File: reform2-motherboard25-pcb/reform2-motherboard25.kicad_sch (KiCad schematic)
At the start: 44 parts, among them J15 Conn_01x33, J18 Conn_01x03_Male, J19 JTAG, J20 Conn_01x03_Male, SW3 SW_DIP_x01, SW5 SW_DIP_x04, SW6 SW_Push, U1 Nitrogen8M_SOM

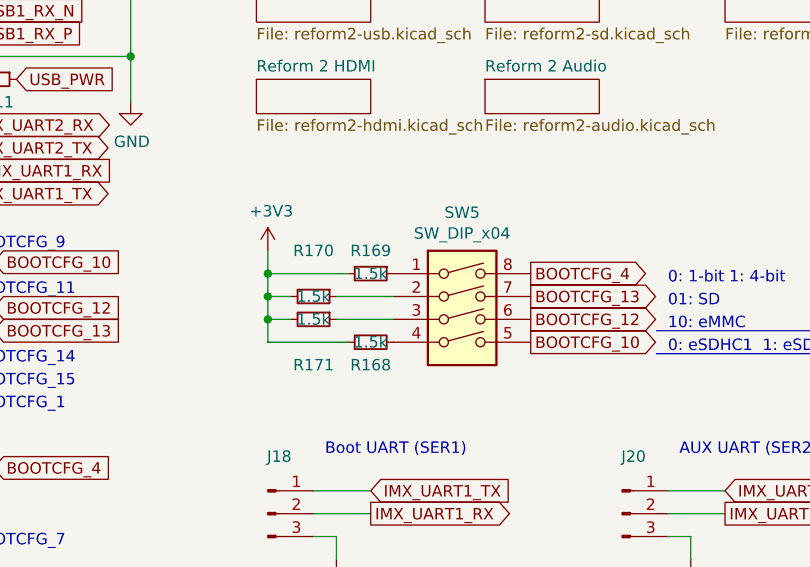
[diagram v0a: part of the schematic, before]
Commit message: motherboard 2.5 snapshot: fully routed and cleaned up
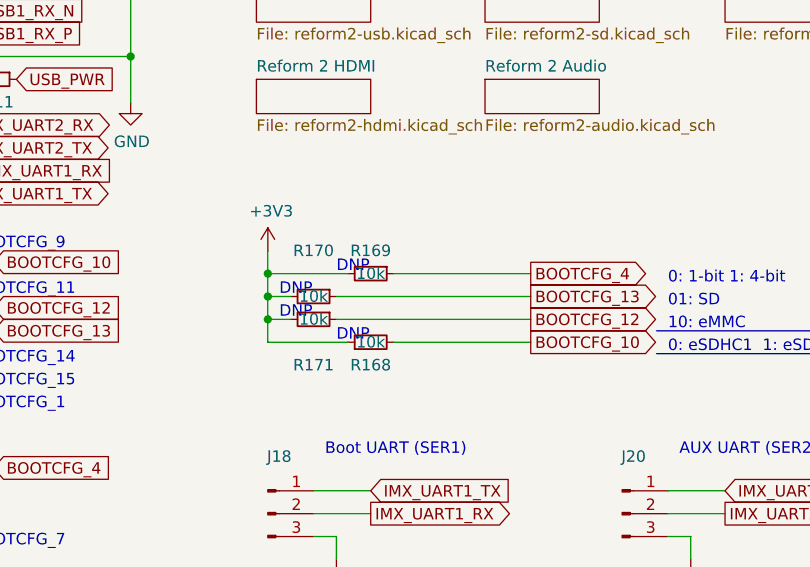
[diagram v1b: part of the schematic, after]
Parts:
- removed SW5: SW_DIP_x04, Button_Switch_SMD:SW_DIP_SPSTx04_Slide_Copal_CHS-04B_W7.62mm_P1.27mm, symbol Switch:SW_DIP_x04
- R113, R115, R117, R118, R119: Distributor Mouser -> (none)
- R168, R169, R170, R171: value 1.5k -> 10k; DNP (none) -> y; Distributor Mouser -> (none); Manufacturer_No RC0603FR-071K5L -> RC0603FR-0710KL
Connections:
- net BOOTCFG_10: now also R168.2
- net BOOTCFG_12: now also R171.1
- net BOOTCFG_13: now also R170.1
- net BOOTCFG_4: now also R169.1
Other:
- note added: "DNP"
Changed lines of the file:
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@@
     (stroke (width 0) (type default) (color 0 0 0 0))
   )
-  (wire (pts (xy 125.73 193.04) (xy 119.38 193.04))
+  (wire (pts (xy 119.38 193.04) (xy 140.97 193.04))
     (stroke (width 0) (type default) (color 0 0 0 0))
   )
@@
     (stroke (width 0) (type default) (color 0 0 0 0))
   )
+  (wire (pts (xy 125.73 198.12) (xy 140.97 198.12))
+    (stroke (width 0) (type default) (color 0 0 0 0))
+  )
   (wire (pts (xy 127 30.48) (xy 127 46.99))
     (stroke (width 0) (type default) (color 0 0 0 0))
@@
     (stroke (width 0) (type default) (color 0 0 0 0))
   )
+  (wire (pts (xy 125.73 190.5) (xy 140.97 190.5))
+    (stroke (width 0) (type default) (color 0 0 0 0))
+  )
   (wire (pts (xy 123.19 214.63) (xy 116.84 214.63))
     (stroke (width 0) (type default) (color 0 0 0 0))
@@
     (stroke (width 0) (type default) (color 0 0 0 0))
   )
-  (wire (pts (xy 125.73 195.58) (xy 119.38 195.58))
+  (wire (pts (xy 119.38 195.58) (xy 140.97 195.58))
     (stroke (width 0) (type default) (color 0 0 0 0))
   )
@@
     (effects (font (size 1.27 1.27)) (justify left bottom))
   )
+  (text "DNP" (at 119.38 198.12 0)
+    (effects (font (size 1.27 1.27)) (justify left bottom))
+  )
+  (text "DNP" (at 113.03 193.04 0)
+    (effects (font (size 1.27 1.27)) (justify left bottom))
+  )
+  (text "DNP" (at 113.03 195.58 0)
+    (effects (font (size 1.27 1.27)) (justify left bottom))
+  )
   (text "BOOTCFG_15" (at 78.74 203.2 0)
     (effects (font (size 1.27 1.27)) (justify left bottom))
   )
+  (text "DNP" (at 119.38 190.5 0)
+    (effects (font (size 1.27 1.27)) (justify left bottom))
+  )
   (text "NOSTUFF" (at 123.19 22.86 0)
     (effects (font (size 1.27 1.27)) (justify left bottom))
@@
       (effects (font (size 1.27 1.27)) hide)
     )
-    (property "Distributor" "Mouser" (id 7) (at 165.1 240.03 0)
+    (property "Distributor" "" (id 7) (at 165.1 240.03 0)
       (effects (font (size 1.27 1.27)) hide)
     )
@@
       (effects (font (size 1.27 1.27)) hide)
     )
-    (property "Distributor" "Mouser" (id 7) (at 107.95 240.03 0)
+    (property "Distributor" "" (id 7) (at 107.95 240.03 0)
       (effects (font (size 1.27 1.27)) hide)
     )
@@
     (in_bom yes) (on_board yes)
     (property "Reference" "R169" (id 0) (at 123.19 187.96 90))
-    (property "Value" "1.5k" (id 1) (at 123.19 190.5 90))
+    (property "Value" "10k" (id 1) (at 123.19 190.5 90))
     (property "Footprint" "Resistor_SMD:R_0603_1608Metric" (id 2) (at 123.19 190.5 0)
       (effects (font (size 1.27 1.27)) hide)
@@
       (effects (font (size 1.27 1.27)) hide)
     )
-    (property "Manufacturer_No" "RC0603FR-071K5L" (id 5) (at 123.19 190.5 0)
+    (property "Manufacturer_No" "RC0603FR-0710KL" (id 5) (at 123.19 190.5 0)
       (effects (font (size 1.27 1.27)) hide)
     )
@@
       (effects (font (size 1.27 1.27)) hide)
     )
-    (property "Distributor" "Mouser" (id 7) (at 123.19 190.5 0)
+    (property "Distributor" "" (id 7) (at 123.19 190.5 0)
+      (effects (font (size 1.27 1.27)) hide)
+    )
+    (property "DNP" "y" (id 8) (at 123.19 190.5 0)
       (effects (font (size 1.27 1.27)) hide)
     )
@@
     (in_bom yes) (on_board yes)
     (property "Reference" "R170" (id 0) (at 116.84 187.96 90))
-    (property "Value" "1.5k" (id 1) (at 116.84 193.04 90))
+    (property "Value" "10k" (id 1) (at 116.84 193.04 90))
     (property "Footprint" "Resistor_SMD:R_0603_1608Metric" (id 2) (at 116.84 193.04 0)
       (effects (font (size 1.27 1.27)) hide)
@@
       (effects (font (size 1.27 1.27)) hide)
     )
-    (property "Manufacturer_No" "RC0603FR-071K5L" (id 5) (at 116.84 193.04 0)
+    (property "Manufacturer_No" "RC0603FR-0710KL" (id 5) (at 116.84 193.04 0)
       (effects (font (size 1.27 1.27)) hide)
     )
@@
       (effects (font (size 1.27 1.27)) hide)
     )
-    (property "Distributor" "Mouser" (id 7) (at 116.84 193.04 0)
+    (property "Distributor" "" (id 7) (at 116.84 193.04 0)
+      (effects (font (size 1.27 1.27)) hide)
+    )
+    (property "DNP" "y" (id 8) (at 116.84 193.04 0)
       (effects (font (size 1.27 1.27)) hide)
     )
@@
     (in_bom yes) (on_board yes)
     (property "Reference" "R171" (id 0) (at 116.84 200.66 90))
-    (property "Value" "1.5k" (id 1) (at 116.84 195.58 90))
+    (property "Value" "10k" (id 1) (at 116.84 195.58 90))
     (property "Footprint" "Resistor_SMD:R_0603_1608Metric" (id 2) (at 116.84 195.58 0)
       (effects (font (size 1.27 1.27)) hide)
@@
       (effects (font (size 1.27 1.27)) hide)
     )
-    (property "Manufacturer_No" "RC0603FR-071K5L" (id 5) (at 116.84 195.58 0)
+    (property "Manufacturer_No" "RC0603FR-0710KL" (id 5) (at 116.84 195.58 0)
       (effects (font (size 1.27 1.27)) hide)
     )
@@
       (effects (font (size 1.27 1.27)) hide)
     )
-    (property "Distributor" "Mouser" (id 7) (at 116.84 195.58 0)
+    (property "Distributor" "" (id 7) (at 116.84 195.58 0)
       (effects (font (size 1.27 1.27)) hide)
     )
-    (pin "1")
-    (pin "2")
-  )
-  (symbol (lib_id "Switch:SW_DIP_x04") (at 133.35 195.58 0) (unit 1)
-    (in_bom yes) (on_board yes)
-    (property "Reference" "SW5" (id 0) (at 133.35 183.7182 0))
-    (property "Value" "SW_DIP_x04" (id 1) (at 133.35 186.0296 0))
-    (property "Footprint" "Button_Switch_SMD:SW_DIP_SPSTx04_Slide_Copal_CHS-04B_W7.62mm_P1.27mm" (id 2) (at 133.35 195.58 0)
-      (effects (font (size 1.27 1.27)) hide)
-    )
-    (property "Datasheet" "" (id 3) (at 133.35 195.58 0)
-      (effects (font (size 1.27 1.27)) hide)
-    )
-    (property "Manufacturer" "Diptronics" (id 4) (at 133.35 195.58 0)
-      (effects (font (size 1.27 1.27)) hide)
-    )
-    (property "Manufacturer_No" "DHA-04TQ" (id 5) (at 133.35 195.58 0)
-      (effects (font (size 1.27 1.27)) hide)
-    )
-    (property "Checked" "y" (id 6) (at 133.35 195.58 0)
-      (effects (font (size 1.27 1.27)) hide)
-    )
-    (property "Distributor" "Mouser" (id 7) (at 133.35 195.58 0)
+    (property "DNP" "y" (id 8) (at 116.84 195.58 0)
       (effects (font (size 1.27 1.27)) hide)
     )
     (pin "1")
     (pin "2")
-    (pin "3")
-    (pin "4")
-    (pin "5")
-    (pin "6")
-    (pin "7")
-    (pin "8")
   )
   (symbol (lib_id "Device:R_Small") (at 123.19 198.12 90) (unit 1)
     (in_bom yes) (on_board yes)
     (property "Reference" "R168" (id 0) (at 123.19 200.66 90))
-    (property "Value" "1.5k" (id 1) (at 123.19 198.12 90))
+    (property "Value" "10k" (id 1) (at 123.19 198.12 90))
     (property "Footprint" "Resistor_SMD:R_0603_1608Metric" (id 2) (at 123.19 198.12 0)
       (effects (font (size 1.27 1.27)) hide)
@@
       (effects (font (size 1.27 1.27)) hide)
     )
-    (property "Manufacturer_No" "RC0603FR-071K5L" (id 5) (at 123.19 198.12 0)
+    (property "Manufacturer_No" "RC0603FR-0710KL" (id 5) (at 123.19 198.12 0)
       (effects (font (size 1.27 1.27)) hide)
     )
@@
       (effects (font (size 1.27 1.27)) hide)
     )
-    (property "Distributor" "Mouser" (id 7) (at 123.19 198.12 0)
+    (property "Distributor" "" (id 7) (at 123.19 198.12 0)
+      (effects (font (size 1.27 1.27)) hide)
+    )
+    (property "DNP" "y" (id 8) (at 123.19 198.12 0)
       (effects (font (size 1.27 1.27)) hide)
     )
@@
       (effects (font (size 1.27 1.27)) hide)
     )
-    (property "Distributor" "Mouser" (id 7) (at 119.38 27.94 0)
+    (property "Distributor" "" (id 7) (at 119.38 27.94 0)
       (effects (font (size 1.27 1.27)) hide)
     )
@@
       (effects (font (size 1.27 1.27)) hide)
     )
-    (property "Distributor" "Mouser" (id 7) (at 127 27.94 0)
+    (property "Distributor" "" (id 7) (at 127 27.94 0)
       (effects (font (size 1.27 1.27)) hide)
     )
@@
       (effects (font (size 1.27 1.27)) hide)
     )
-    (property "Distributor" "Mouser" (id 7) (at 134.62 27.94 0)
+    (property "Distributor" "" (id 7) (at 134.62 27.94 0)
       (effects (font (size 1.27 1.27)) hide)
     )
@@
     )
     (path "/00000000-0000-0000-0000-00005e437433"
-      (reference "R168") (unit 1) (value "1.5k") (footprint "Resistor_SMD:R_0603_1608Metric")
+      (reference "R168") (unit 1) (value "10k") (footprint "Resistor_SMD:R_0603_1608Metric")
     )
     (path "/00000000-0000-0000-0000-00005e2c5325"
-      (reference "R169") (unit 1) (value "1.5k") (footprint "Resistor_SMD:R_0603_1608Metric")
+      (reference "R169") (unit 1) (value "10k") (footprint "Resistor_SMD:R_0603_1608Metric")
     )
     (path "/00000000-0000-0000-0000-00005e2d1326"
-      (reference "R170") (unit 1) (value "1.5k") (footprint "Resistor_SMD:R_0603_1608Metric")
+      (reference "R170") (unit 1) (value "10k") (footprint "Resistor_SMD:R_0603_1608Metric")
     )
     (path "/00000000-0000-0000-0000-00005e31432e"
-      (reference "R171") (unit 1) (value "1.5k") (footprint "Resistor_SMD:R_0603_1608Metric")
+      (reference "R171") (unit 1) (value "10k") (footprint "Resistor_SMD:R_0603_1608Metric")
     )
     (path "/00000000-0000-0000-0000-00005cc81028/00000000-0000-0000-0000-0000613df725"
@@
       (reference "SW3") (unit 1) (value "SW_DIP_x01") (footprint "Button_Switch_SMD:SW_DIP_SPSTx01_Slide_Omron_A6S-110x_W8.9mm_P2.54mm")
     )
-    (path "/00000000-0000-0000-0000-00005e3779c3"
-      (reference "SW5") (unit 1) (value "SW_DIP_x04") (footprint "Button_Switch_SMD:SW_DIP_SPSTx04_Slide_Copal_CHS-04B_W7.62mm_P1.27mm")
-    )
     (path "/00000000-0000-0000-0000-00005dbc8bec"

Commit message: motherboard25: r-1 snapshot, ordered for test bringup
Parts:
- R113, R115, R117, R118, R119, R168, R169, R170, R171: Distributor (none) -> Mouser
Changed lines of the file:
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@@
       (effects (font (size 1.27 1.27)) hide)
     )
-    (property "Distributor" "" (id 7) (at 165.1 240.03 0)
+    (property "Distributor" "Mouser" (id 7) (at 165.1 240.03 0)
       (effects (font (size 1.27 1.27)) hide)
     )
@@
       (effects (font (size 1.27 1.27)) hide)
     )
-    (property "Distributor" "" (id 7) (at 107.95 240.03 0)
+    (property "Distributor" "Mouser" (id 7) (at 107.95 240.03 0)
       (effects (font (size 1.27 1.27)) hide)
     )
@@
       (effects (font (size 1.27 1.27)) hide)
     )
-    (property "Distributor" "" (id 7) (at 123.19 190.5 0)
+    (property "Distributor" "Mouser" (id 7) (at 123.19 190.5 0)
       (effects (font (size 1.27 1.27)) hide)
     )
@@
       (effects (font (size 1.27 1.27)) hide)
     )
-    (property "Distributor" "" (id 7) (at 116.84 193.04 0)
+    (property "Distributor" "Mouser" (id 7) (at 116.84 193.04 0)
       (effects (font (size 1.27 1.27)) hide)
     )
@@
       (effects (font (size 1.27 1.27)) hide)
     )
-    (property "Distributor" "" (id 7) (at 116.84 195.58 0)
+    (property "Distributor" "Mouser" (id 7) (at 116.84 195.58 0)
       (effects (font (size 1.27 1.27)) hide)
     )
@@
       (effects (font (size 1.27 1.27)) hide)
     )
-    (property "Distributor" "" (id 7) (at 123.19 198.12 0)
+    (property "Distributor" "Mouser" (id 7) (at 123.19 198.12 0)
       (effects (font (size 1.27 1.27)) hide)
     )
@@
       (effects (font (size 1.27 1.27)) hide)
     )
-    (property "Distributor" "" (id 7) (at 119.38 27.94 0)
+    (property "Distributor" "Mouser" (id 7) (at 119.38 27.94 0)
       (effects (font (size 1.27 1.27)) hide)
     )
@@
       (effects (font (size 1.27 1.27)) hide)
     )
-    (property "Distributor" "" (id 7) (at 127 27.94 0)
+    (property "Distributor" "Mouser" (id 7) (at 127 27.94 0)
       (effects (font (size 1.27 1.27)) hide)
     )
@@
       (effects (font (size 1.27 1.27)) hide)
     )
-    (property "Distributor" "" (id 7) (at 134.62 27.94 0)
+    (property "Distributor" "Mouser" (id 7) (at 134.62 27.94 0)
       (effects (font (size 1.27 1.27)) hide)
     )
@@
       (reference "#PWR0259") (unit 1) (value "GND") (footprint "")
     )
+    (path "/00000000-0000-0000-0000-00005cc81028/a6962170-aaca-4dae-92ab-e32d1208aa58"
+      (reference "#PWR0260") (unit 1) (value "GND") (footprint "")
+    )
     (path "/00000000-0000-0000-0000-00005cc81028/00000000-0000-0000-0000-0000616517a7/00000000-0000-0000-0000-000066ae38d8"
       (reference "BT1") (unit 1) (value "CR1220") (footprint "Battery:BatteryHolder_Keystone_3000_1x12mm")
@@
     )
     (path "/00000000-0000-0000-0000-00005d06a2fd/9af1cb30-120c-4bd0-9692-20a1323b5bd7"
-      (reference "J12") (unit 1) (value "Conn_02x06_Odd_Even") (footprint "Connector_PinHeader_1.00mm:PinHeader_2x06_P1.00mm_Vertical_SMD")
+      (reference "J12") (unit 1) (value "Conn_02x08_Odd_Even") (footprint "Connector_PinHeader_1.00mm:PinHeader_2x08_P1.00mm_Vertical_SMD")
     )
     (path "/00000000-0000-0000-0000-00005cc81028/00000000-0000-0000-0000-00005f00ed51"
@@
     )
     (path "/00000000-0000-0000-0000-00005cc81028/00000000-0000-0000-0000-00005d74f9c5"
-      (reference "R79") (unit 1) (value "0") (footprint "Resistor_SMD:R_0603_1608Metric")
+      (reference "R79") (unit 1) (value "100k NTC") (footprint "Resistor_SMD:R_0603_1608Metric")
     )
     (path "/00000000-0000-0000-0000-00005cc81028/00000000-0000-0000-0000-000061ec7b4b"
@@
       (reference "R85") (unit 1) (value "10k") (footprint "Resistor_SMD:R_0603_1608Metric")
     )
+    (path "/00000000-0000-0000-0000-00005cc81028/07fb6cb0-ebdc-4ba2-b22b-899fe29e117f"
+      (reference "R86") (unit 1) (value "100k") (footprint "Resistor_SMD:R_0603_1608Metric")
+    )
+    (path "/00000000-0000-0000-0000-00005cc81028/6e154ce1-0a68-4826-b5a7-263e5ce7cb40"
+      (reference "R87") (unit 1) (value "10k") (footprint "Resistor_SMD:R_0603_1608Metric")
+    )
+    (path "/00000000-0000-0000-0000-00005cc81028/c67aad6d-47f7-4799-bea1-dd33431c5f11"
+      (reference "R88") (unit 1) (value "0") (footprint "Resistor_SMD:R_0603_1608Metric")
+    )
+    (path "/00000000-0000-0000-0000-00005cc81028/e27d426e-9660-4ada-8e20-4434c3ef9296"
+      (reference "R89") (unit 1) (value "0") (footprint "Resistor_SMD:R_0603_1608Metric")
+    )
     (path "/00000000-0000-0000-0000-00005d06a2fd/00000000-0000-0000-0000-00005d950f53"
